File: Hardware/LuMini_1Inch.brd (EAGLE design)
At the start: 28.7 x 28.7 mm, 35 parts, among them J1 DOUBLE_LED_PAD, J2 DOUBLE_LED_PAD, J3 DOUBLE_LED_PAD, J4 DOUBLE_LED_PAD

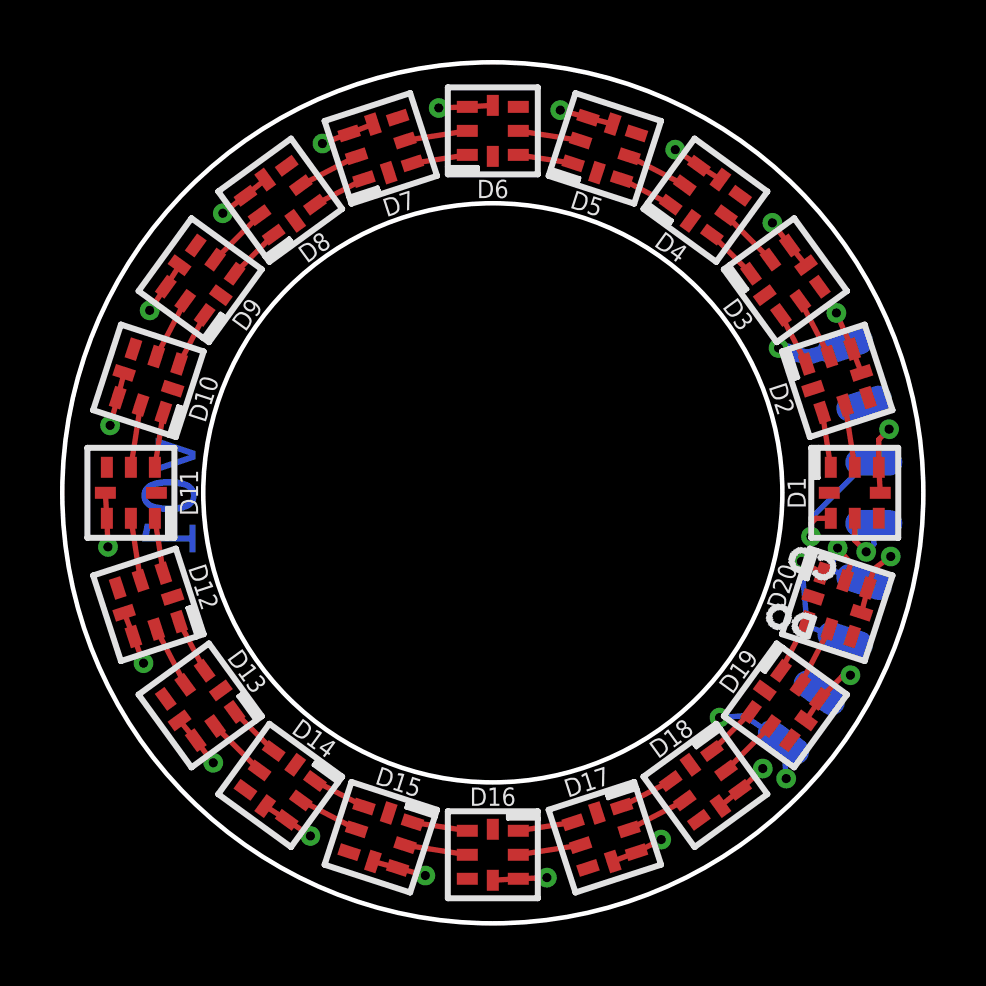
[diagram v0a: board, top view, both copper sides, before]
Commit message: Cleaning repo, changing name, pre review
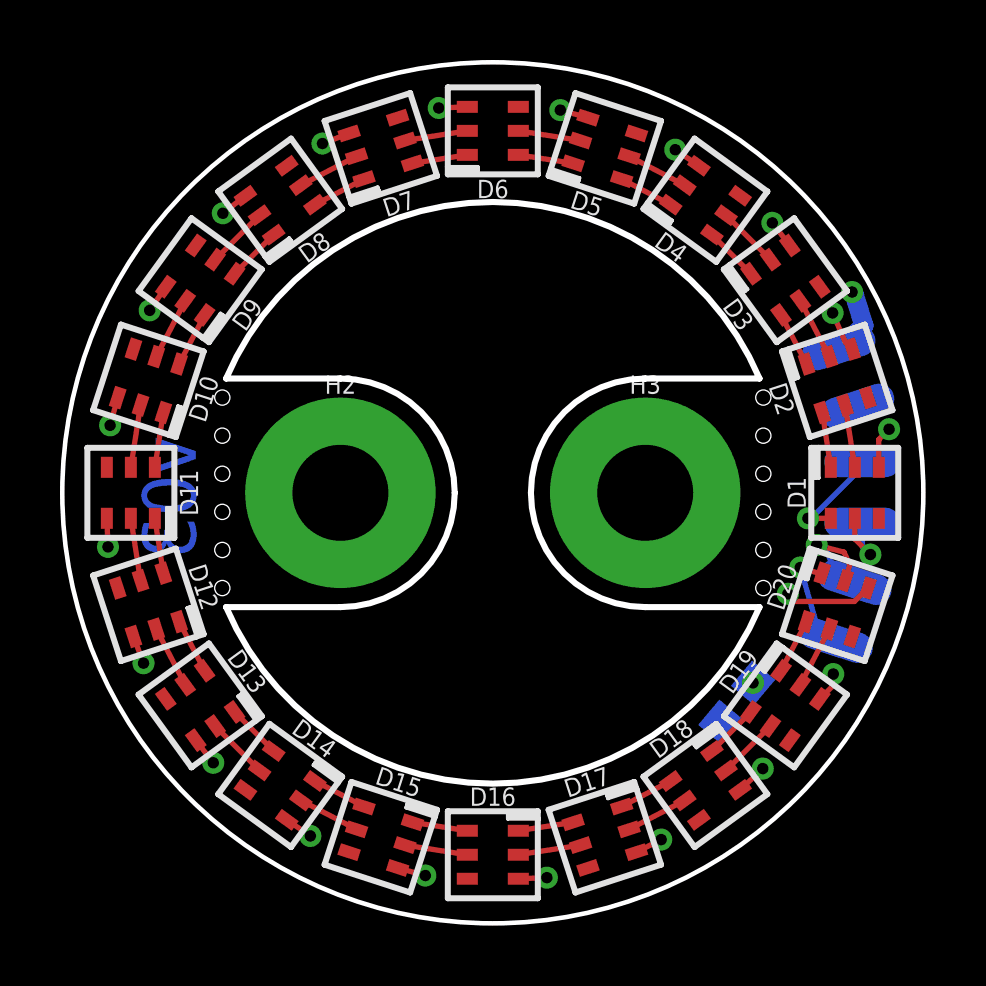
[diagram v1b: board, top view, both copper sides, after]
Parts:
- removed J3: DOUBLE_LED_PAD, Andy:DOUBLELEDPAD
- removed U$3: (no value), buzzard_labels (25):5V6
- removed U$6: (no value), buzzard_labels (25):G4
- added C1: 4.7uF, SparkFun-Capacitors:0603
- added H2, H3: STANDOFF_ELECTRICALSTANDOFF-ELECTRICAL-NOTHERMALS, SparkFun-Hardware:STANDOFF-ELECTRICAL-NOTHERMALS
- U$1: device buzzard_labels (22):CHROMADOT5 -> buzzard_labels (2):LUMINI0
- moved FRAME1 70.3 mm to (-10.2, -6.35)
- moved U$8 2.46 mm to (25.9, 14.3), flipped to the bottom, turned to 288 degrees
- moved U$7 2.35 mm to (25.3, 12.4), flipped to the bottom, turned to 288 degrees
- moved U$4 2.25 mm to (25.0, 18.9), turned to 252 degrees
- moved U$9 2.21 mm to (25.7, 15.5), turned to 270 degrees
- moved U$10 2.19 mm to (25.7, 17.4), turned to 270 degrees
- moved U$5 2.12 mm to (24.5, 20.5), turned to 252 degrees
- moved U$1 0.65 mm to (18.5, 27.2)
- moved J2 0.38 mm to (27.6, 15.3)
- moved J4 0.32 mm to (27.0, 11.3)
- moved J1 0.24 mm to (27.1, 19.1)
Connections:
- net 5V: now also C1.1; no longer D1.VDDPAD, D10.VDDPAD, D11.VDDPAD, D12.VDDPAD, D13.VDDPAD, D14.VDDPAD, D15.VDDPAD, D16.VDDPAD, D17.VDDPAD, D18.VDDPAD, D19.VDDPAD, D2.VDDPAD, D20.VDDPAD, D3.VDDPAD, D4.VDDPAD, D5.VDDPAD, D6.VDDPAD, D7.VDDPAD, D8.VDDPAD, D9.VDDPAD, J3.P$2
- net GND: now also C1.2, H2.P1, H3.P1; no longer D1.GNDPAD, D10.GNDPAD, D11.GNDPAD, D12.GNDPAD, D13.GNDPAD, D14.GNDPAD, D15.GNDPAD, D16.GNDPAD, D17.GNDPAD, D18.GNDPAD, D19.GNDPAD, D2.GNDPAD, D20.GNDPAD, D3.GNDPAD, D4.GNDPAD, D5.GNDPAD, D6.GNDPAD, D7.GNDPAD, D8.GNDPAD, D9.GNDPAD, J3.P$1
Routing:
- net 5V: track 38.0 -> 22.1 mm
- net GND: track 5.96 -> 2.34 mm, vias 3 -> 2
- net N$3: track 4.76 -> 3.52 mm
- net N$41: track 3.16 -> 3.90 mm
- net N$42: track 4.32 -> 3.72 mm
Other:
- outline, holes or cut-outs redrawn
- board text added: "Andy England"
- board text added: "v03"
- board text removed: "v01"
